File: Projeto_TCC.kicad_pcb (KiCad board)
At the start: 2 copper layers, 58 parts, among them J1 Screw_Terminal_01x02, J2 Jack-DC, J3 Conn_01x15, J4 Conn_01x15, J5 Conn_01x04, J6 Conn_01x04, J7 Conn_01x04, J8 Conn_01x04, K1 AY1RC2, K2 AY1RC2, Q1 BC337, Q2 BC337, Q3 IRF540N, U1 PC817, U2 PC817, U3 LM324, U4 L7805, U5 L7812

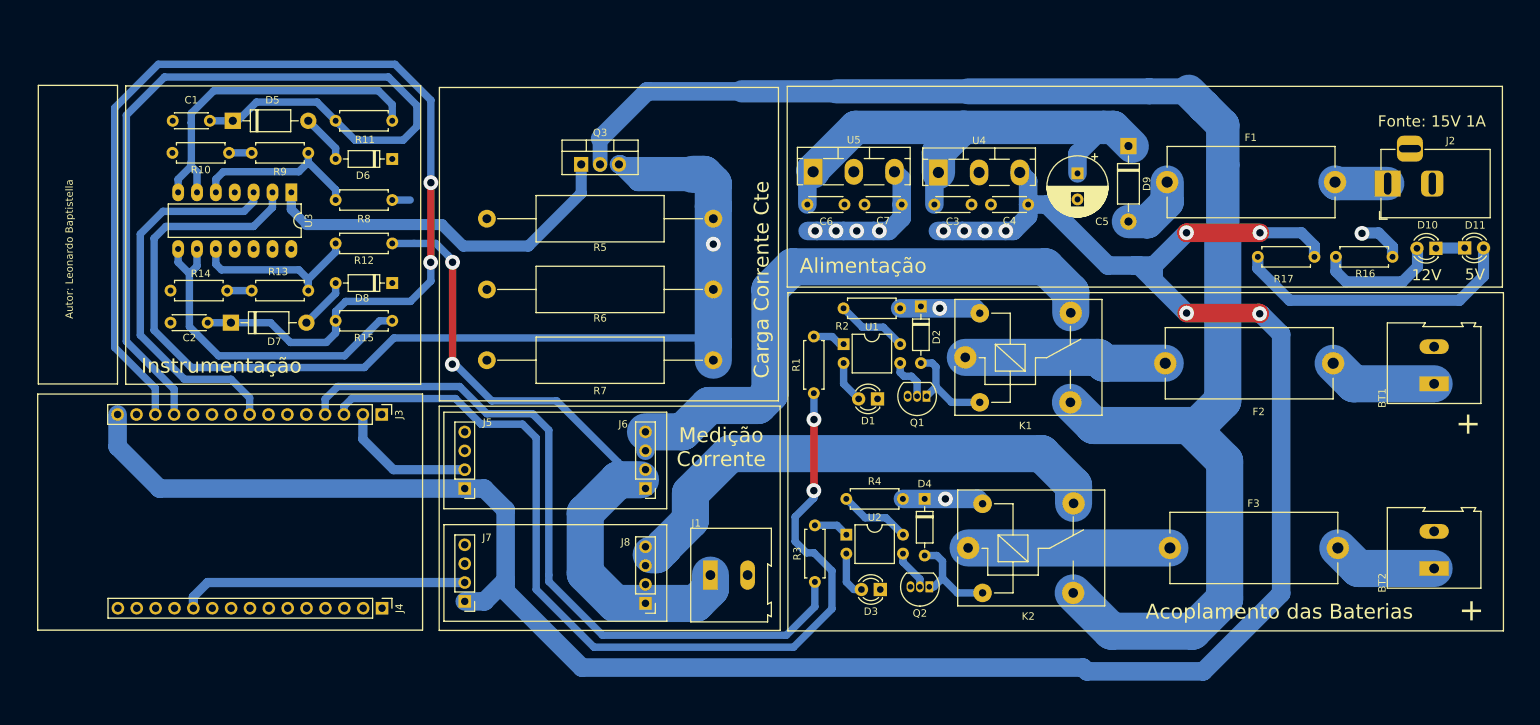
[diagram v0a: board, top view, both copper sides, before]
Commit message: Battery tester TCC
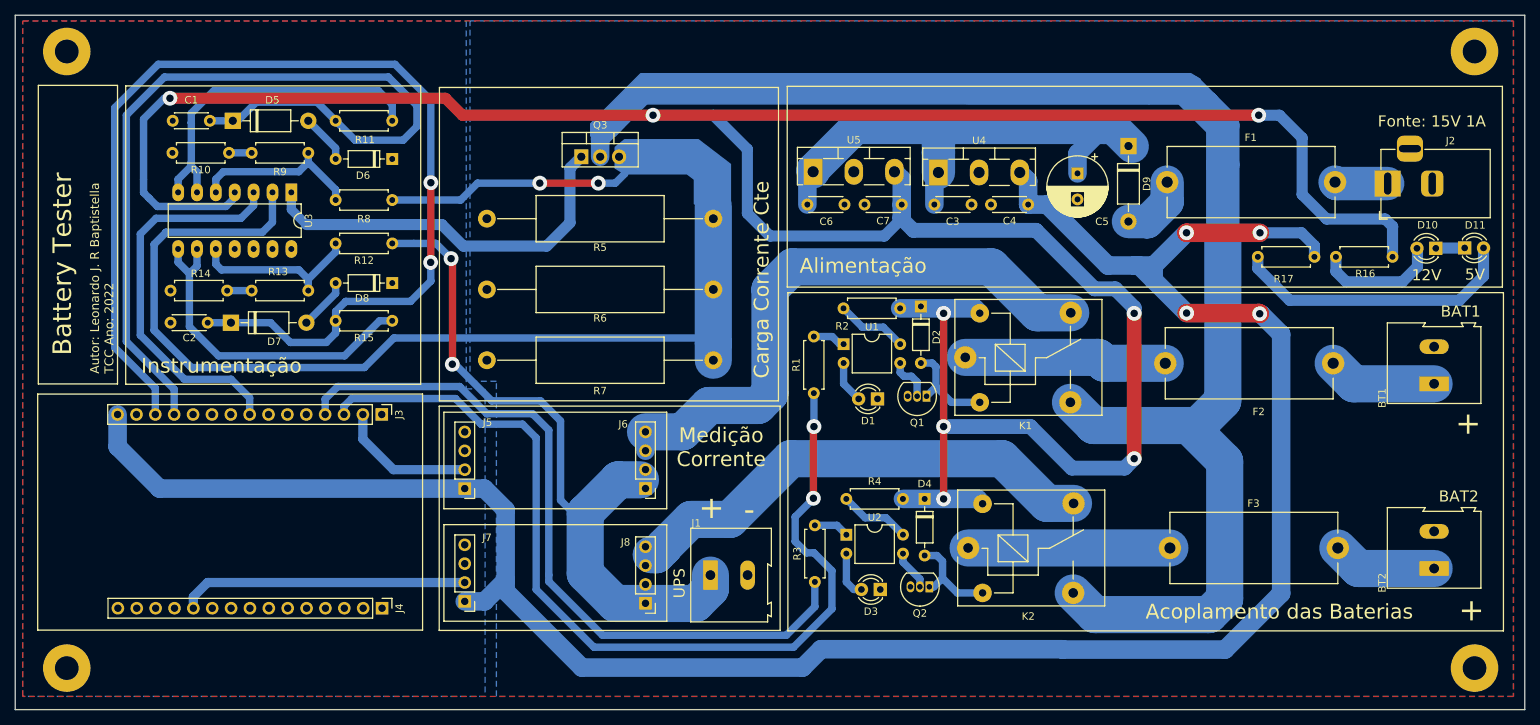
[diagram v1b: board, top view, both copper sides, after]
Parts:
- added REF**: MountingHole_3.2mm_M3_Pad, MountingHole:MountingHole_3.2mm_M3_Pad, F.Cu at (58.5, 60.0)
- added REF**: MountingHole_3.2mm_M3_Pad, MountingHole:MountingHole_3.2mm_M3_Pad, F.Cu at (58.5, 143.0)
- added REF**: MountingHole_3.2mm_M3_Pad, MountingHole:MountingHole_3.2mm_M3_Pad, F.Cu at (248.0, 143.0)
- added REF**: MountingHole_3.2mm_M3_Pad, MountingHole:MountingHole_3.2mm_M3_Pad, F.Cu at (248.0, 60.0)
- moved Q3 1.03 mm to (127.8, 74.2)
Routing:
- net +12V: track 68.4 -> 412.0 mm, vias 7 -> 8
- net +5V: track 317.1 -> 301.9 mm, vias 9 -> 4
- net V_IN1: track 204.8 -> 218.0 mm, vias 1 -> 2
- net LOAD: track 229.4 -> 223.3 mm
- net AMP2: track 68.8 -> 64.7 mm
- net Net-(Q3-Pad1): track 50.2 -> 52.7 mm
- net +UPS: track 92.3 -> 94.1 mm
- net AMP1: track 81.4 -> 79.8 mm
- net Net-(C3-Pad1): track 72.8 -> 72.0 mm
- added copper zone on B.Cu, net GND
- added copper zone on F.Cu, net GND
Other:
- board outline added: 203.2 x 93.5 mm
- board text added: "-"
- board text added: "Autor: Leonardo J. R Baptistella TCC Ano: 2022"
- board text added: "BAT1"
- board text added: "BAT2"
- board text added: "Battery Tester"
- board text added: "UPS"
- board text removed: "Autor: Leonardo Baptistella"
